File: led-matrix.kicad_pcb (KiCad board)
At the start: 2 copper layers, 102.5 x 53 mm, 138 parts

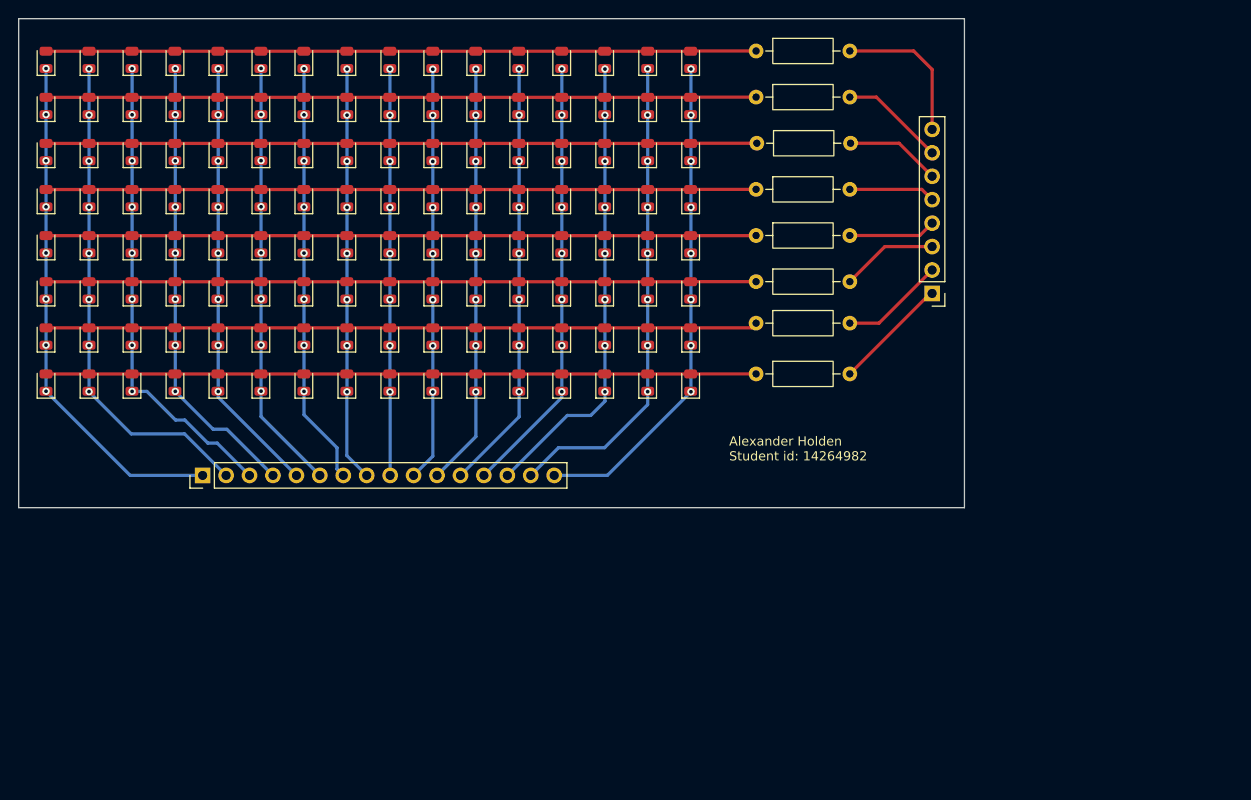
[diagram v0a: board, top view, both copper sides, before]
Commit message: hey
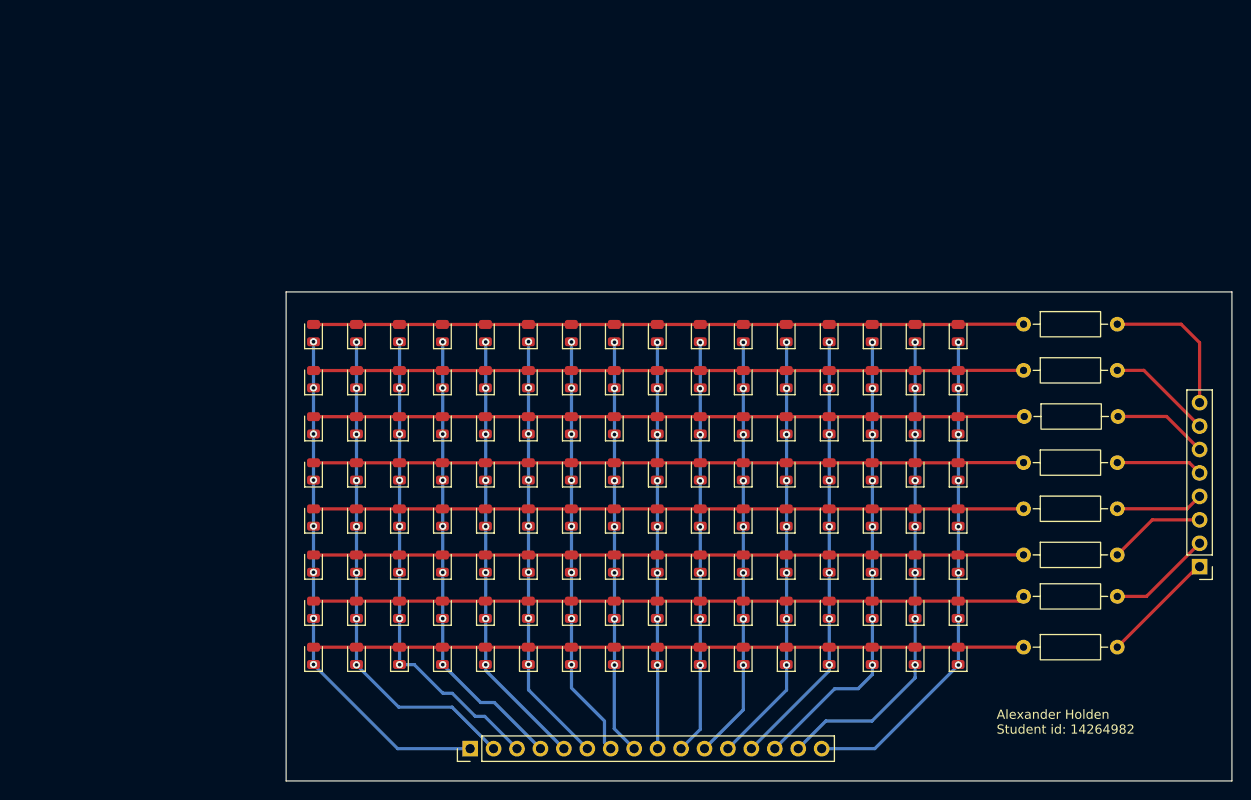
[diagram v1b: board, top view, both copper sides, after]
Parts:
- moved D10 41.4 mm to (144.4, 65.6)
- moved D11 41.4 mm to (149.0, 65.6)
- moved D13 41.4 mm to (158.3, 65.6)
- moved D14 41.4 mm to (163.0, 65.6)
- moved D15 41.4 mm to (167.7, 65.6)
- moved D16 41.4 mm to (172.3, 65.6)
- moved D23 41.4 mm to (130.4, 70.6)
- moved D24 41.4 mm to (135.1, 70.6)
- moved D25 41.4 mm to (139.7, 70.6)
- moved D26 41.4 mm to (144.4, 70.6)
- moved D27 41.4 mm to (149.0, 70.6)
- moved D29 41.4 mm to (158.3, 70.6)
- moved D30 41.4 mm to (163.0, 70.6)
- moved D31 41.4 mm to (167.7, 70.6)
- moved D32 41.4 mm to (172.3, 70.6)
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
